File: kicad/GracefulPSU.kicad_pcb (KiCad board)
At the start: 2 copper layers, 91.4 x 105.4 mm, 73 parts, among them J1 +12V in1, J10 +5V, J11 0V, J2 +12V in2, J3 0v, J4 Conn_02x20_Odd_Even, J5 LED-, J6 LED+, J7 Sw, J8 Sw, J9 +5Vu, Q1 CSD19505KCS, Q2 IRF7319, Q3 CSD19505KCS, U1 LM358, U2 LM22678TJ-ADJ

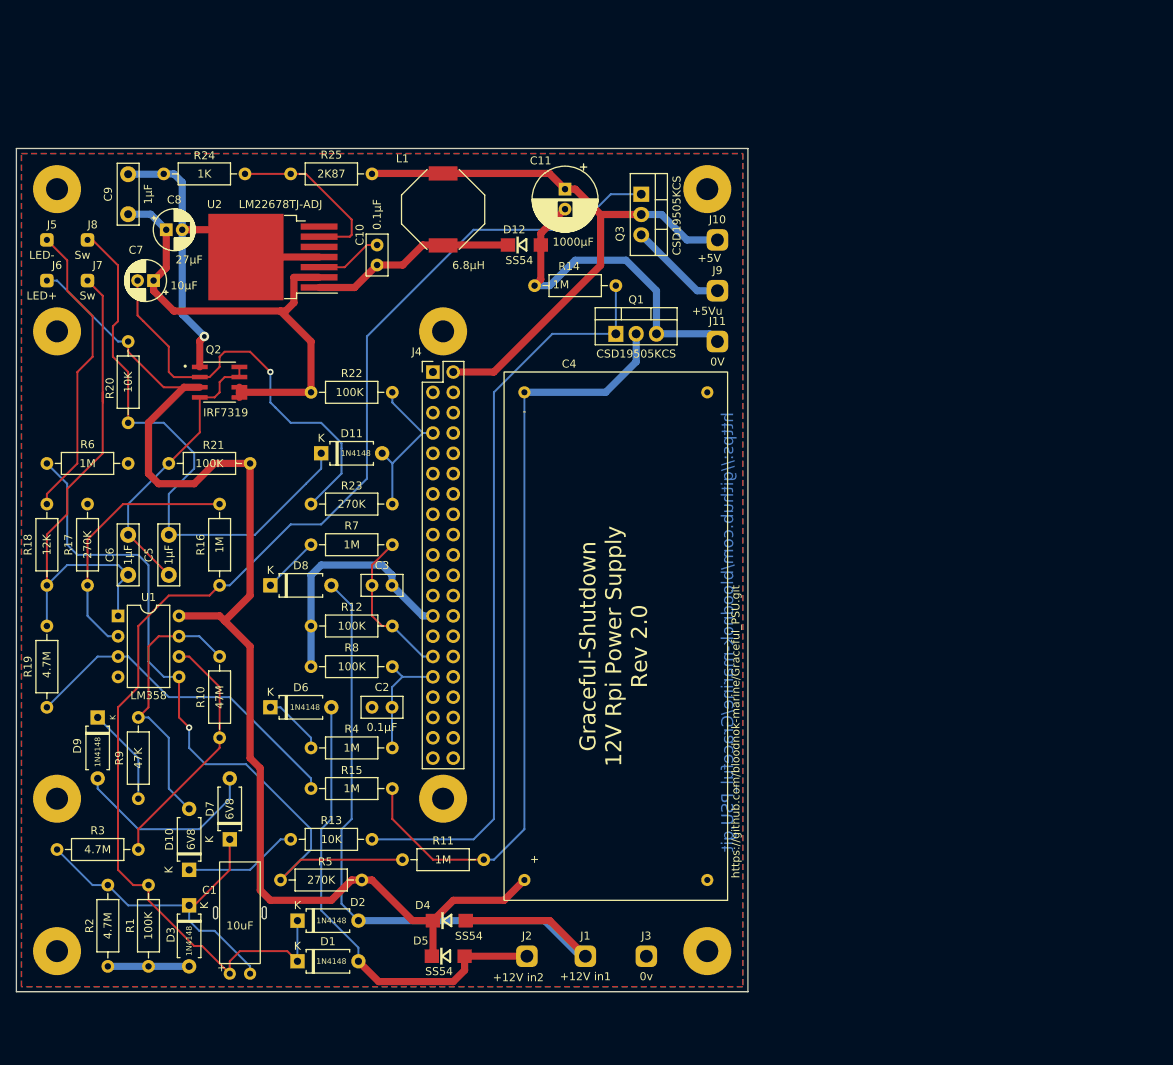
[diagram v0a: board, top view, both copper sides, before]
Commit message: Release of version sent for pcb manufacture.
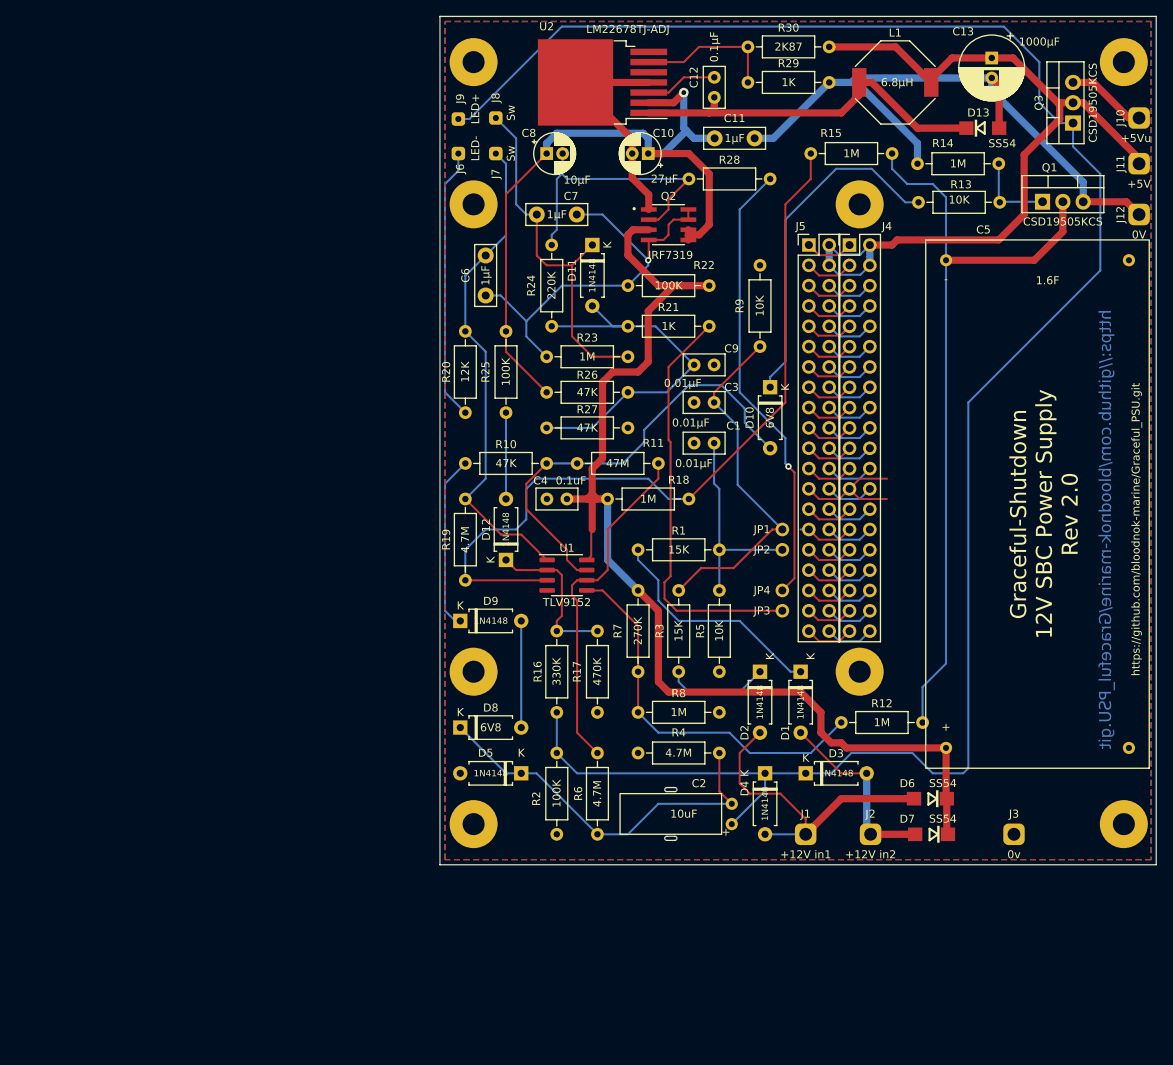
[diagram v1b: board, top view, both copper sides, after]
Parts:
- added C12: 0.1μF, Capacitor_THT:C_Disc_D5.0mm_W2.5mm_P2.50mm, F.Cu at (130.4, 44.5)
- added C13: 1000μF, Capacitor_THT:CP_Radial_D8.0mm_P2.50mm, F.Cu at (165.1, 42.0)
- added D13: SS54, my_extras:DO-214AC, F.Cu at (164.0, 50.8)
- added J12: 0V, my_extras:SolderConnector - HighCurrent, F.Cu at (183.5, 61.6)
- added JP1: Jumper, my_extras:Half-Jumper, F.Cu at (138.9, 101.0)
- added JP2: Jumper, my_extras:Half-Jumper, F.Cu at (138.9, 103.5)
- added JP3: Jumper, my_extras:Half-Jumper, F.Cu at (138.9, 111.1)
- added JP4: Jumper, my_extras:Half-Jumper, F.Cu at (138.9, 108.6)
- added R26: 47K, Resistor_THT:R_Axial_DIN0207_L6.3mm_D2.5mm_P10.16mm_Horizontal, F.Cu at (119.6, 83.8)
- added R27: 47K, Resistor_THT:R_Axial_DIN0207_L6.3mm_D2.5mm_P10.16mm_Horizontal, F.Cu at (109.5, 88.3)
- added R28: 10K, Resistor_THT:R_Axial_DIN0207_L6.3mm_D2.5mm_P10.16mm_Horizontal, F.Cu at (127.2, 57.1)
- added R29: 1K, Resistor_THT:R_Axial_DIN0207_L6.3mm_D2.5mm_P10.16mm_Horizontal, F.Cu at (134.6, 45.1)
- added R30: 2K87, Resistor_THT:R_Axial_DIN0207_L6.3mm_D2.5mm_P10.16mm_Horizontal, F.Cu at (134.6, 40.6)
- C1: value 10uF -> 0.01μF; footprint my_extras:Capacitor_THT_HorizRadial_D5_P2_H12 -> Capacitor_THT:C_Disc_D5.0mm_W2.5mm_P2.50mm
- C10: value 0.1μF -> 27μF; footprint Capacitor_THT:C_Disc_D5.0mm_W2.5mm_P2.50mm -> Capacitor_THT:CP_Radial_D5.0mm_P2.00mm
- C11: value 1000μF -> 1μF; footprint Capacitor_THT:CP_Radial_D8.0mm_P2.50mm -> Capacitor_THT:C_Disc_D7.5mm_W2.5mm_P5.00mm
- C2: value 0.1μF -> 10uF; footprint Capacitor_THT:C_Disc_D5.0mm_W2.5mm_P2.50mm -> my_extras:Capacitor_THT_HorizRadial_D5_P2_H12
- C3: value 0.1μF -> 0.01μF
- C4: value 1.6F -> 0.1uF; footprint my_extras:SuperCapacitor Module -> Capacitor_THT:C_Disc_D5.0mm_W2.5mm_P2.50mm
- C5: value 1μF -> 1.6F; footprint Capacitor_THT:C_Disc_D7.5mm_W2.5mm_P5.00mm -> my_extras:SuperCapacitor Module
- C7: value 10μF -> 1μF; footprint Capacitor_THT:CP_Radial_D5.0mm_P2.00mm -> Capacitor_THT:C_Disc_D7.5mm_W2.5mm_P5.00mm
- C8: value 27μF -> 10μF
- C9: value 1μF -> 0.01μF; footprint Capacitor_THT:C_Disc_D7.5mm_W2.5mm_P5.00mm -> Capacitor_THT:C_Disc_D5.0mm_W2.5mm_P2.50mm
- D12, D4, D5: value SS54 -> 1N4148; footprint my_extras:DO-214AC -> Diode_THT:D_A-405_P7.62mm_Horizontal
- D6: value 1N4148 -> SS54; footprint Diode_THT:D_A-405_P7.62mm_Horizontal -> my_extras:DO-214AC
- D7: value 6V8 -> SS54; footprint Diode_THT:D_A-405_P7.62mm_Horizontal -> my_extras:DO-214AC
- D8: value 1N4148 -> 6V8
- J10: value +5V -> +5Vu
- J11: value 0V -> +5V
- J4: value Conn_02x20_Odd_Even -> Conn_02x20
- J5: value LED- -> Conn_02x20; footprint my_extras:SolderConnector -> Connector_PinHeader_2.54mm:PinHeader_2x20_P2.54mm_Vertical
- J6: value LED+ -> LED-
- J9: value +5Vu -> LED+; footprint my_extras:SolderConnector - HighCurrent -> my_extras:SolderConnector
- R1: value 100K -> 15K
- R10: value 47M -> 47K
- R11: value 1M -> 47M
- R12, R8: value 100K -> 1M
- R16: value 1M -> 330K
- R17: value 270K -> 470K
- R18: value 12K -> 1M
- R2: value 4.7M -> 100K
- R20: value 10K -> 12K
- R21: value 100K -> 1K
- R23: value 270K -> 1M
- R24: value 1K -> 220K
- R25: value 2K87 -> 100K
- R3: value 4.7M -> 15K
- R4, R6: value 1M -> 4.7M
- R5: value 270K -> 10K
- R7: value 1M -> 270K
- R9: value 47K -> 10K
- U1: value LM358 -> TLV9152; footprint Package_DIP:DIP-8_W7.62mm -> Package_SO:SOIC-8_3.9x4.9mm_P1.27mm
- moved R13 111.8 mm to (155.9, 60.1)
- moved C5 107.4 mm to (169.5, 110.5), turned to 180 degrees
- moved R9 102.4 mm to (136.1, 67.9), turned to -90 degrees
- moved R15 101.0 mm to (152.6, 54.0)
- moved J5 95.3 mm to (142.2, 65.4)
- moved D10 94.4 mm to (137.4, 83.2), turned to -90 degrees
- moved D7 87.7 mm to (157.6, 139.1), turned to 180 degrees
- moved C1 87.3 mm to (127.9, 90.2)
- moved D6 83.3 mm to (157.4, 134.6), turned to 180 degrees
- moved R6 83.0 mm to (115.8, 139.1), turned to 90 degrees
- moved R3 80.8 mm to (126.0, 118.7), turned to 90 degrees
- moved D3 78.8 mm to (141.8, 131.4), turned to 0 degrees
- moved R1 74.2 mm to (120.9, 103.5), turned to 0 degrees
- moved C9 73.2 mm to (127.9, 80.4), turned to 0 degrees
- moved D1 72.6 mm to (141.2, 118.7), turned to -90 degrees
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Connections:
- C1 pad 1: Net-(C1-Pad1) -> GND
- C10 pad 2: Net-(C10-Pad2) -> GND
- C11 pad 1: Net-(C11-Pad1) -> Net-(C10-Pad1)
- C2 pad 1: GND -> Net-(C2-Pad1)
- C4 pad 2: Net-(C4-Pad2) -> GND
- C5 pad 1: Net-(C5-Pad1) -> Net-(C4-Pad1)
- C6 pad 1: Net-(C5-Pad1) -> Net-(C6-Pad1)
- C7 pad 1: Net-(C7-Pad1) -> Net-(C6-Pad1)
- C8 pad 1: Net-(C7-Pad1) -> Net-(C10-Pad1)
- C8 pad 2: GND -> Net-(C8-Pad2)
- C9 pad 1: Net-(C7-Pad1) -> Net-(D11-Pad2)
- D1 pad 1: Net-(C1-Pad1) -> Net-(D1-Pad1)
- D11 pad 1: Net-(C5-Pad2) -> Net-(C7-Pad2)
- D12 pad 1: Net-(C10-Pad2) -> Net-(D12-Pad1)
- D12 pad 2: GND -> Net-(D12-Pad2)
- D2 pad 1: Net-(C1-Pad1) -> Net-(D2-Pad1)
- D3 pad 1: Net-(C1-Pad2) -> Net-(C2-Pad1)
- D3 pad 2: GND -> Net-(D1-Pad2)
- D4 pad 1: Net-(C4-Pad1) -> Net-(C2-Pad1)
- D5 pad 1: Net-(C4-Pad1) -> Net-(C2-Pad2)
- D5 pad 2: Net-(D1-Pad2) -> GND
- D6 pad 1: Net-(D6-Pad1) -> Net-(C4-Pad1)
- D6 pad 2: Net-(D1-Pad2) -> Net-(D2-Pad2)
- D7 pad 1: Net-(C1-Pad2) -> Net-(C4-Pad1)
- D7 pad 2: Net-(D7-Pad2) -> Net-(D1-Pad2)
- D8 pad 1: Net-(D8-Pad1) -> Net-(C2-Pad2)
- D8 pad 2: Net-(D2-Pad2) -> Net-(D8-Pad2)
- D9 pad 2: Net-(D7-Pad2) -> Net-(D8-Pad2)
- J10 pad 1: Net-(C11-Pad1) -> Net-(J10-Pad1)
- J11 pad 1: GND -> +5V
- J4 pad 1: unconnected-(J4-Pad1) -> Net-(J4-Pad1)
- J4 pad 10: unconnected-(J4-Pad10) -> Net-(J4-Pad10)
- J4 pad 11: unconnected-(J4-Pad11) -> Net-(J4-Pad11)
- J4 pad 12: unconnected-(J4-Pad12) -> Net-(J4-Pad12)
- J4 pad 13: unconnected-(J4-Pad13) -> Net-(J4-Pad13)
- J4 pad 14: unconnected-(J4-Pad14) -> GND
- J4 pad 15: unconnected-(J4-Pad15) -> Net-(J4-Pad15)
- J4 pad 16: unconnected-(J4-Pad16) -> Net-(J4-Pad16)
- J4 pad 17: unconnected-(J4-Pad17) -> Net-(J4-Pad17)
- J4 pad 18: unconnected-(J4-Pad18) -> Net-(J4-Pad18)
- J4 pad 19: unconnected-(J4-Pad19) -> Net-(J4-Pad19)
- J4 pad 2: Net-(C11-Pad1) -> +5V
- J4 pad 20: unconnected-(J4-Pad20) -> GND
- J4 pad 21: unconnected-(J4-Pad21) -> Net-(J4-Pad21)
- J4 pad 22: unconnected-(J4-Pad22) -> Net-(J4-Pad22)
- J4 pad 23: unconnected-(J4-Pad23) -> Net-(J4-Pad23)
- J4 pad 24: unconnected-(J4-Pad24) -> Net-(J4-Pad24)
- J4 pad 26: unconnected-(J4-Pad26) -> Net-(J4-Pad26)
- J4 pad 27: unconnected-(J4-Pad27) -> Net-(J4-Pad27)
- J4 pad 28: unconnected-(J4-Pad28) -> Net-(J4-Pad28)
- J4 pad 29: Net-(C3-Pad1) -> Net-(J4-Pad29)
- J4 pad 3: unconnected-(J4-Pad3) -> Net-(J4-Pad3)
- J4 pad 30: unconnected-(J4-Pad30) -> GND
- J4 pad 31: Net-(C2-Pad2) -> Net-(J4-Pad31)
- J4 pad 32: unconnected-(J4-Pad32) -> Net-(J4-Pad32)
- J4 pad 33: unconnected-(J4-Pad33) -> Net-(J4-Pad33)
- J4 pad 34: unconnected-(J4-Pad34) -> GND
- J4 pad 35: unconnected-(J4-Pad35) -> Net-(J4-Pad35)
- J4 pad 36: unconnected-(J4-Pad36) -> Net-(JP3-Pad2)
- J4 pad 37: unconnected-(J4-Pad37) -> Net-(J4-Pad37)
- J4 pad 38: unconnected-(J4-Pad38) -> Net-(J4-Pad38)
- J4 pad 39: unconnected-(J4-Pad39) -> GND
- J4 pad 4: unconnected-(J4-Pad4) -> +5V
- J4 pad 40: unconnected-(J4-Pad40) -> Net-(J4-Pad40)
- J4 pad 5: unconnected-(J4-Pad5) -> Net-(J4-Pad5)
- J4 pad 6: unconnected-(J4-Pad6) -> GND
- J4 pad 7: Net-(D11-Pad2) -> Net-(J4-Pad7)
- J4 pad 8: unconnected-(J4-Pad8) -> Net-(J4-Pad8)
- J4 pad 9: unconnected-(J4-Pad9) -> GND
- J5 pad 1: Net-(J5-Pad1) -> Net-(J4-Pad1)
- J6 pad 1: Net-(C4-Pad1) -> Net-(J6-Pad1)
- J8 pad 1: Net-(C5-Pad2) -> Net-(C7-Pad2)
- J9 pad 1: Net-(J9-Pad1) -> Net-(C2-Pad1)
- L1 pad 1: Net-(C10-Pad2) -> Net-(C12-Pad2)
- L1 pad 2: Net-(C11-Pad1) -> +5V
- Q1 pad 2: Net-(C4-Pad2) -> Net-(C5-Pad2)
- Q2 pad 2: Net-(C7-Pad2) -> Net-(C8-Pad2)
- Q2 pad 4: Net-(C5-Pad1) -> Net-(C6-Pad1)
- Q2 pad 5: Net-(C7-Pad1) -> Net-(C10-Pad1)
- Q2 pad 6: Net-(C7-Pad1) -> Net-(C10-Pad1)
- Q2 pad 7: Net-(C5-Pad1) -> Net-(C6-Pad1)
- Q2 pad 8: Net-(C5-Pad1) -> Net-(C6-Pad1)
- Q3 pad 1: Net-(C1-Pad1) -> Net-(C2-Pad1)
- Q3 pad 2: Net-(C11-Pad1) -> +5V
- Q3 pad 3: Net-(J9-Pad1) -> Net-(J10-Pad1)
- R1 pad 1: Net-(C1-Pad1) -> Net-(D1-Pad1)
- R1 pad 2: GND -> Net-(C1-Pad2)
- R10 pad 1: Net-(R10-Pad1) -> Net-(D9-Pad1)
- R11 pad 2: Net-(C4-Pad2) -> Net-(D10-Pad2)
- R12 pad 1: GND -> Net-(R12-Pad1)
- R12 pad 2: Net-(C3-Pad1) -> Net-(C5-Pad2)
- R15 pad 1: Net-(C4-Pad2) -> Net-(C5-Pad2)
- R16 pad 1: Net-(C1-Pad1) -> Net-(C2-Pad1)
- R16 pad 2: Net-(R16-Pad2) -> Net-(D12-Pad1)
- R17 pad 1: Net-(R16-Pad2) -> Net-(D12-Pad1)
- R18 pad 1: Net-(C6-Pad2) -> Net-(C4-Pad1)
- R18 pad 2: Net-(J5-Pad1) -> Net-(R15-Pad2)
- R2 pad 1: Net-(C1-Pad2) -> Net-(C2-Pad1)
- R20 pad 1: Net-(C4-Pad1) -> Net-(J6-Pad1)
- R20 pad 2: Net-(C5-Pad2) -> Net-(C6-Pad2)
- R21 pad 1: Net-(C4-Pad1) -> Net-(D11-Pad2)
- R21 pad 2: Net-(C5-Pad1) -> Net-(JP3-Pad1)
- R22 pad 1: Net-(C7-Pad1) -> Net-(C4-Pad1)
- R22 pad 2: Net-(D11-Pad2) -> Net-(C6-Pad1)
- R23 pad 1: Net-(D11-Pad2) -> Net-(C6-Pad1)
- R24 pad 1: Net-(R24-Pad1) -> Net-(C8-Pad2)
- R24 pad 2: GND -> Net-(D11-Pad2)
- R25 pad 1: Net-(R24-Pad1) -> Net-(C10-Pad1)
- R25 pad 2: Net-(C11-Pad1) -> Net-(D12-Pad2)
- R3 pad 1: Net-(C1-Pad2) -> Net-(D2-Pad1)
- R3 pad 2: Net-(R10-Pad1) -> Net-(C3-Pad1)
- R4 pad 1: Net-(D6-Pad1) -> Net-(C2-Pad2)
- R4 pad 2: Net-(C2-Pad2) -> GND
- R5 pad 1: Net-(C4-Pad1) -> GND
- R5 pad 2: Net-(R11-Pad1) -> Net-(C1-Pad2)
- R6 pad 1: Net-(R11-Pad1) -> Net-(C2-Pad2)
- R6 pad 2: GND -> Net-(R11-Pad1)
- R7 pad 1: Net-(D8-Pad1) -> Net-(C4-Pad1)
- R7 pad 2: Net-(C3-Pad1) -> Net-(R12-Pad1)
- R8 pad 1: GND -> Net-(R12-Pad1)
- R8 pad 2: Net-(C2-Pad2) -> GND
- R9 pad 1: Net-(D9-Pad1) -> GND
- R9 pad 2: Net-(D10-Pad2) -> Net-(C3-Pad1)
- U1 pad 2: Net-(R16-Pad2) -> Net-(D12-Pad1)
- U1 pad 5: Net-(R11-Pad1) -> Net-(R12-Pad1)
- U1 pad 6: Net-(R10-Pad1) -> Net-(R11-Pad1)
- U2 pad 1: Net-(C10-Pad2) -> Net-(C12-Pad2)
- U2 pad 2: Net-(C7-Pad1) -> Net-(C10-Pad1)
- U2 pad 3: Net-(C10-Pad1) -> Net-(C12-Pad1)
- U2 pad 6: Net-(R24-Pad1) -> Net-(R29-Pad1)
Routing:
- net Net-(C2-Pad1): track 0.00 -> 246.5 mm
- net Net-(C1-Pad1): track 163.8 -> 0.00 mm
- net +5V: track 0.00 -> 101.8 mm
- net Net-(C4-Pad2): track 97.7 -> 0.00 mm
- net Net-(Q1-Pad1): track 93.9 -> 10.00 mm
- net Net-(C10-Pad1): track 8.39 -> 89.8 mm, vias 0 -> 1
- net Net-(C11-Pad1): track 76.9 -> 0.00 mm
- net Net-(C7-Pad1): track 61.2 -> 0.00 mm
- net Net-(JP4-Pad1): track 0.00 -> 56.5 mm, vias 0 -> 1
- net Net-(R15-Pad2): track 43.2 -> 98.4 mm
- net Net-(C6-Pad1): track 0.00 -> 52.6 mm, vias 0 -> 1
- net Net-(JP3-Pad1): track 0.00 -> 51.9 mm
- net Net-(D2-Pad2): track 91.4 -> 39.9 mm
- net Net-(R11-Pad1): track 92.2 -> 43.5 mm, vias 1 -> 0
- net Net-(R12-Pad1): track 0.00 -> 48.1 mm
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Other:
- board size 91.4 x 105.4 mm -> 89.5 x 106 mm
- board text added: "Graceful-Shutdown 12V SBC Power Supply Rev 2.0"
- board text removed: "Graceful-Shutdown 12V Rpi Power Supply Rev 2.0"

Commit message: Prep for release to github.
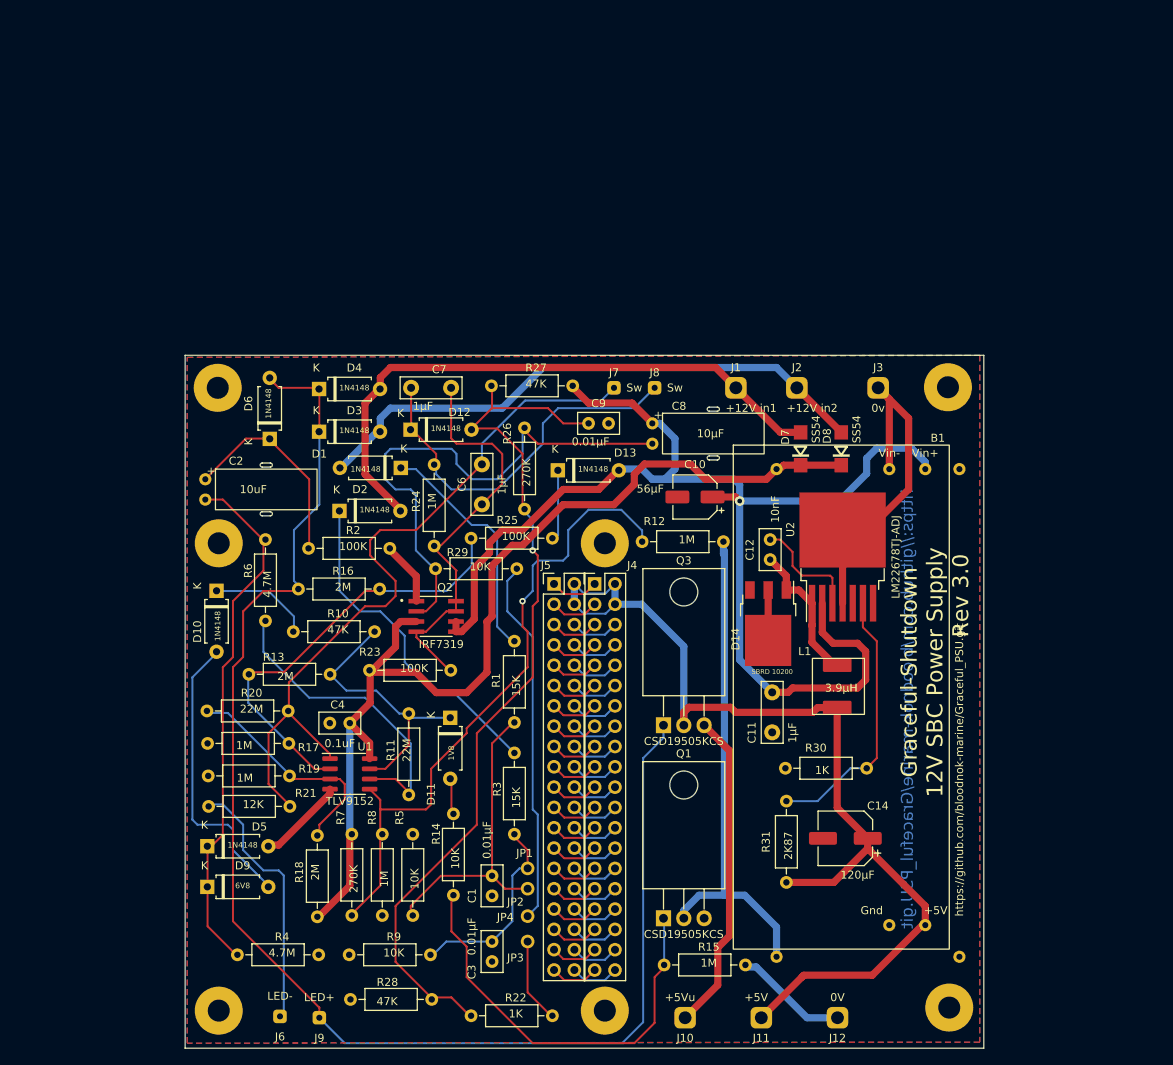
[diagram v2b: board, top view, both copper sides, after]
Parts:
- removed C13: 1000μF, Capacitor_THT:CP_Radial_D8.0mm_P2.50mm
- removed H7: , 
- added B1: PSU_Board, my_extras:Buck Power Supply Board, F.Cu at (146.3, 123.9)
- added C14: 120μF, Capacitor_SMD:CP_Elec_6.3x5.9, F.Cu at (146.8, 139.6)
- added D14: SBRD 10200, Package_TO_SOT_SMD:TO-252-3_TabPin2, F.Cu at (137.1, 112.7)
- added R31: 2K87, my_extras:my_resistor_6.3_2.5_10.16, F.Cu at (139.2, 135.0)
- C10: value 27μF -> 56μF; footprint Capacitor_THT:CP_Radial_D5.0mm_P2.00mm -> Capacitor_SMD:CP_Elec_5x5.3
- C12: value 0.1μF -> 10nF
- C5: moved to B.Cu
- C8: footprint Capacitor_THT:CP_Radial_D5.0mm_P2.00mm -> my_extras:Capacitor_THT_HorizRadial_D5_P2_H12
- D1, D12, D2, D3, D4, D5: footprint Diode_THT:D_A-405_P7.62mm_Horizontal -> my_extras:my_diode_7.62_h
- D10: value 6V8 -> 1N4148; footprint Diode_THT:D_A-405_P7.62mm_Horizontal -> my_extras:my_diode_7.62_h
- D11: value 1N4148 -> 1V8; footprint Diode_THT:D_A-405_P7.62mm_Horizontal -> my_extras:my_diode_7.62_h
- D13, D6: value SS54 -> 1N4148; footprint my_extras:DO-214AC -> my_extras:my_diode_7.62_h
- D8: value 6V8 -> SS54; footprint Diode_THT:D_A-405_P7.62mm_Horizontal -> my_extras:DO-214AC
- D9: value 1N4148 -> 6V8; footprint Diode_THT:D_A-405_P7.62mm_Horizontal -> my_extras:my_diode_7.62_h
- L1: value 6.8μH -> 3.9μH; footprint Inductor_SMD:L_Bourns-SRU1028_10.0x10.0mm -> my_extras:Shenzhen MWSA0604S
- Q1, Q3: footprint Package_TO_SOT_THT:TO-220-3_Vertical -> Package_TO_SOT_THT:TO-220-3_Horizontal_TabDown
- R1, R10, R12, R15, R2, R25, R27, R3, R4, R5, R6, R7, R8, R9: footprint Resistor_THT:R_Axial_DIN0207_L6.3mm_D2.5mm_P10.16mm_Horizontal -> my_extras:my_resistor_6.3_2.5_10.16
- R11: value 47M -> 22M; footprint Resistor_THT:R_Axial_DIN0207_L6.3mm_D2.5mm_P10.16mm_Horizontal -> my_extras:my_resistor_6.3_2.5_10.16
- R13: value 10K -> 2M; footprint Resistor_THT:R_Axial_DIN0207_L6.3mm_D2.5mm_P10.16mm_Horizontal -> my_extras:my_resistor_6.3_2.5_10.16
- R14: value 1M -> 10K; footprint Resistor_THT:R_Axial_DIN0207_L6.3mm_D2.5mm_P10.16mm_Horizontal -> my_extras:my_resistor_6.3_2.5_10.16
- R16: value 330K -> 2M; footprint Resistor_THT:R_Axial_DIN0207_L6.3mm_D2.5mm_P10.16mm_Horizontal -> my_extras:my_resistor_6.3_2.5_10.16
- R17: value 470K -> 1M; footprint Resistor_THT:R_Axial_DIN0207_L6.3mm_D2.5mm_P10.16mm_Horizontal -> my_extras:my_resistor_6.3_2.5_10.16
- R18: value 1M -> 2M; footprint Resistor_THT:R_Axial_DIN0207_L6.3mm_D2.5mm_P10.16mm_Horizontal -> my_extras:my_resistor_6.3_2.5_10.16
- R19: value 4.7M -> 1M; footprint Resistor_THT:R_Axial_DIN0207_L6.3mm_D2.5mm_P10.16mm_Horizontal -> my_extras:my_resistor_6.3_2.5_10.16
- R20: value 12K -> 22M; footprint Resistor_THT:R_Axial_DIN0207_L6.3mm_D2.5mm_P10.16mm_Horizontal -> my_extras:my_resistor_6.3_2.5_10.16
- R21: value 1K -> 12K; footprint Resistor_THT:R_Axial_DIN0207_L6.3mm_D2.5mm_P10.16mm_Horizontal -> my_extras:my_resistor_6.3_2.5_10.16
- R22: value 100K -> 1K; footprint Resistor_THT:R_Axial_DIN0207_L6.3mm_D2.5mm_P10.16mm_Horizontal -> my_extras:my_resistor_6.3_2.5_10.16
- R23: value 1M -> 100K; footprint Resistor_THT:R_Axial_DIN0207_L6.3mm_D2.5mm_P10.16mm_Horizontal -> my_extras:my_resistor_6.3_2.5_10.16
- R24: value 220K -> 1M; footprint Resistor_THT:R_Axial_DIN0207_L6.3mm_D2.5mm_P10.16mm_Horizontal -> my_extras:my_resistor_6.3_2.5_10.16
- R26: value 47K -> 270K; footprint Resistor_THT:R_Axial_DIN0207_L6.3mm_D2.5mm_P10.16mm_Horizontal -> my_extras:my_resistor_6.3_2.5_10.16
- R28: value 10K -> 47K; footprint Resistor_THT:R_Axial_DIN0207_L6.3mm_D2.5mm_P10.16mm_Horizontal -> my_extras:my_resistor_6.3_2.5_10.16
- R29: value 1K -> 10K; footprint Resistor_THT:R_Axial_DIN0207_L6.3mm_D2.5mm_P10.16mm_Horizontal -> my_extras:my_resistor_6.3_2.5_10.16
- R30: value 2K87 -> 1K; footprint Resistor_THT:R_Axial_DIN0207_L6.3mm_D2.5mm_P10.16mm_Horizontal -> my_extras:my_resistor_6.3_2.5_10.16
- moved J10 126.0 mm to (126.8, 162.0)
- moved J11 116.7 mm to (136.3, 162.0)
- moved J9 113.7 mm to (81.0, 162.0), turned to 0 degrees
- moved J6 110.1 mm to (76.1, 161.8), turned to 0 degrees
- moved R28 107.3 mm to (95.0, 159.5), turned to 180 degrees
- moved J12 107.2 mm to (145.8, 162.0)
- moved R14 106.3 mm to (97.6, 136.6), turned to -90 degrees
- moved R15 105.6 mm to (124.2, 155.6), turned to 0 degrees
- moved Q1 101.3 mm to (124.1, 149.6)
- moved R9 100.5 mm to (84.9, 154.4), turned to 0 degrees
- moved R22 96.2 mm to (100.1, 162.0), turned to 0 degrees
- moved R13 94.2 mm to (82.3, 118.8), turned to 180 degrees
- moved D6 94.2 mm to (74.7, 89.6), turned to 90 degrees
- moved R30 91.1 mm to (149.4, 130.6), turned to 180 degrees
- moved Q3 91.0 mm to (124.1, 125.4), turned to 0 degrees
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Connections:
- C10 pad 1: Net-(C10-Pad1) -> Net-(B1-Pad3)
- C11 pad 1: Net-(C10-Pad1) -> Net-(B1-Pad3)
- C8 pad 1: Net-(C10-Pad1) -> Net-(B1-Pad3)
- C9 pad 1: Net-(D11-Pad2) -> Net-(C9-Pad1)
- D11 pad 1: Net-(C7-Pad2) -> Net-(D11-Pad1)
- D12 pad 1: Net-(D12-Pad1) -> Net-(C7-Pad2)
- D12 pad 2: Net-(D12-Pad2) -> Net-(C9-Pad1)
- D13 pad 1: Net-(C12-Pad2) -> Net-(D13-Pad1)
- D13 pad 2: GND -> Net-(B1-Pad3)
- D3 pad 1: Net-(C2-Pad1) -> Net-(D3-Pad1)
- D4 pad 1: Net-(C2-Pad1) -> Net-(D3-Pad1)
- D6 pad 1: Net-(C4-Pad1) -> Net-(C2-Pad1)
- D6 pad 2: Net-(D2-Pad2) -> Net-(D3-Pad1)
- D7 pad 2: Net-(D1-Pad2) -> Net-(D2-Pad2)
- D8 pad 1: Net-(C2-Pad2) -> Net-(C4-Pad1)
- D8 pad 2: Net-(D8-Pad2) -> Net-(D1-Pad2)
- D9 pad 1: Net-(D9-Pad1) -> Net-(C2-Pad2)
- D9 pad 2: Net-(D8-Pad2) -> Net-(D10-Pad2)
- J9 pad 1: Net-(C2-Pad1) -> Net-(D3-Pad1)
- Q2 pad 5: Net-(C10-Pad1) -> Net-(B1-Pad3)
- Q2 pad 6: Net-(C10-Pad1) -> Net-(B1-Pad3)
- Q3 pad 1: Net-(C2-Pad1) -> Net-(D3-Pad1)
- R10 pad 1: Net-(D9-Pad1) -> Net-(D10-Pad1)
- R10 pad 2: Net-(D10-Pad2) -> Net-(D11-Pad1)
- R11 pad 2: Net-(D10-Pad2) -> Net-(D11-Pad1)
- R13 pad 1: Net-(D10-Pad1) -> Net-(D11-Pad1)
- R13 pad 2: Net-(Q1-Pad1) -> Net-(R13-Pad2)
- R14 pad 1: Net-(Q1-Pad1) -> Net-(D11-Pad2)
- R14 pad 2: GND -> Net-(Q1-Pad1)
- R15 pad 1: Net-(C5-Pad2) -> Net-(Q1-Pad1)
- R15 pad 2: Net-(R15-Pad2) -> GND
- R16 pad 1: Net-(C2-Pad1) -> Net-(D3-Pad1)
- R16 pad 2: Net-(D12-Pad1) -> Net-(R13-Pad2)
- R17 pad 1: Net-(D12-Pad1) -> Net-(R13-Pad2)
- R18 pad 2: Net-(R15-Pad2) -> Net-(R18-Pad2)
- R19 pad 1: Net-(R15-Pad2) -> Net-(R18-Pad2)
- R19 pad 2: Net-(C6-Pad2) -> GND
- R20 pad 1: Net-(J6-Pad1) -> Net-(R18-Pad2)
- R21 pad 1: Net-(D11-Pad2) -> Net-(J6-Pad1)
- R21 pad 2: Net-(JP3-Pad1) -> Net-(C6-Pad2)
- R22 pad 1: Net-(C4-Pad1) -> Net-(C9-Pad1)
- R22 pad 2: Net-(C6-Pad1) -> Net-(JP3-Pad1)
- R23 pad 1: Net-(C6-Pad1) -> Net-(C4-Pad1)
- R23 pad 2: Net-(C7-Pad2) -> Net-(C6-Pad1)
- R24 pad 1: Net-(C8-Pad2) -> Net-(C6-Pad1)
- R24 pad 2: Net-(D11-Pad2) -> Net-(C7-Pad2)
- R25 pad 1: Net-(C10-Pad1) -> Net-(R13-Pad2)
- R25 pad 2: Net-(D12-Pad2) -> Net-(D13-Pad1)
- R26 pad 1: Net-(D11-Pad2) -> Net-(C8-Pad2)
- R26 pad 2: Net-(C10-Pad1) -> Net-(C9-Pad1)
- R27 pad 1: Net-(D11-Pad2) -> Net-(C9-Pad1)
- R27 pad 2: GND -> Net-(B1-Pad3)
- R28 pad 1: Net-(C8-Pad2) -> Net-(C9-Pad1)
- R28 pad 2: Net-(JP4-Pad1) -> GND
- R29 pad 1: Net-(R29-Pad1) -> Net-(C8-Pad2)
- R29 pad 2: GND -> Net-(JP4-Pad1)
- R30 pad 1: Net-(R29-Pad1) -> Net-(R30-Pad1)
- R30 pad 2: +5V -> GND
- U1 pad 2: Net-(D12-Pad1) -> Net-(R13-Pad2)
- U1 pad 3: Net-(R15-Pad2) -> Net-(R18-Pad2)
- U1 pad 7: Net-(D10-Pad2) -> Net-(D11-Pad1)
- U2 pad 2: Net-(C10-Pad1) -> Net-(B1-Pad3)
- U2 pad 6: Net-(R29-Pad1) -> Net-(R30-Pad1)
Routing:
- net Net-(C2-Pad1): track 246.5 -> 26.1 mm
- net Net-(D3-Pad1): track 0.00 -> 179.1 mm
- net Net-(B1-Pad3): track 0.00 -> 159.3 mm, vias 0 -> 1
- net Net-(C9-Pad1): track 0.00 -> 110.7 mm, vias 0 -> 1
- net Net-(R15-Pad2): track 98.4 -> 0.00 mm
- net Net-(C10-Pad1): track 89.8 -> 0.00 mm, vias 1 -> 0
- net Net-(R13-Pad2): track 0.00 -> 54.1 mm
- net Net-(D1-Pad2): track 23.8 -> 72.2 mm
- net Net-(D11-Pad2): track 47.0 -> 4.45 mm
- net Net-(Q1-Pad1): track 10.00 -> 52.3 mm
- net Net-(JP3-Pad1): track 51.9 -> 10.8 mm
- net GND: track 169.4 -> 132.4 mm
- net Net-(D11-Pad1): track 0.00 -> 36.8 mm
- net Net-(D2-Pad2): track 39.9 -> 75.6 mm
- net Net-(R30-Pad1): track 0.00 -> 33.6 mm
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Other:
- board size 89.5 x 106 mm -> 99.8 x 86.6 mm
- board text added: "Graceful-Shutdown 12V SBC Power Supply Rev 3.0"
- board text removed: "Graceful-Shutdown 12V SBC Power Supply Rev 2.0"
